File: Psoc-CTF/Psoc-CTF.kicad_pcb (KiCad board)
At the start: 2 copper layers, 100 x 100 mm, 123 parts, among them IC1 CY8C4248LQI-BL583, J1 Conn_01x02, J10 Conn_01x20, J11 Conn_01x20, J2 Conn_01x03, J3 Prog, J4 Conn_01x04, J5 USB3076-XX-X_REVC, J6 Header 9x2, J7 Header 9x2, J8 Conn_01x20, J9 Conn_01x20, P1 Power, P2 Analog, P3 Digital, P4 Digital, SW1 FSM4JSMATR, SW2 FSM4JSMATR, SW3 FSM4JSMATR, SW4 FSM4JSMATR, SW5 FSM4JSMATR, U1 AMS1117-5.0, U2 AMS1117-3.3, U3 ESP32-WROOM-32D, U4 FM24C04B-GTR, U5 CY7C65211-24LTXI, Y1 24MHz, Y2 32.768Khz

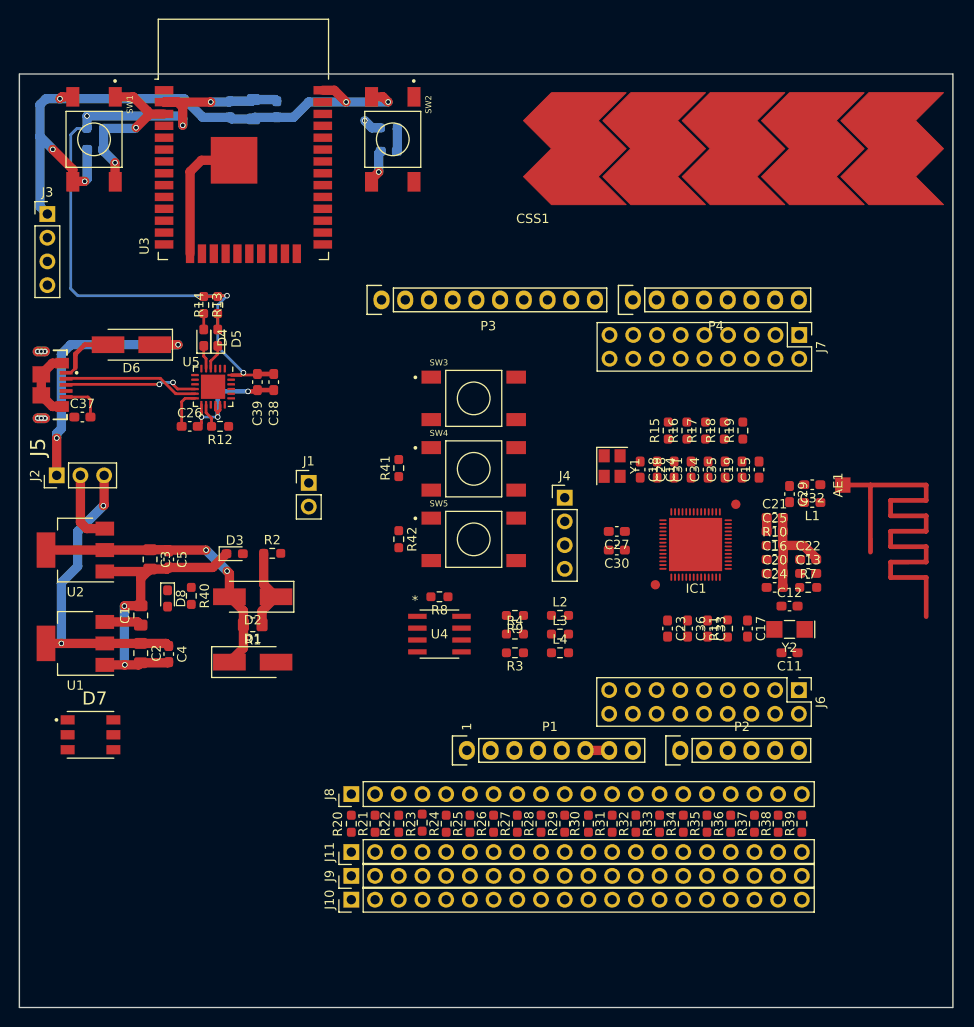
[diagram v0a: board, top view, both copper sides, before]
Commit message: Ruteo Psoc-CTF
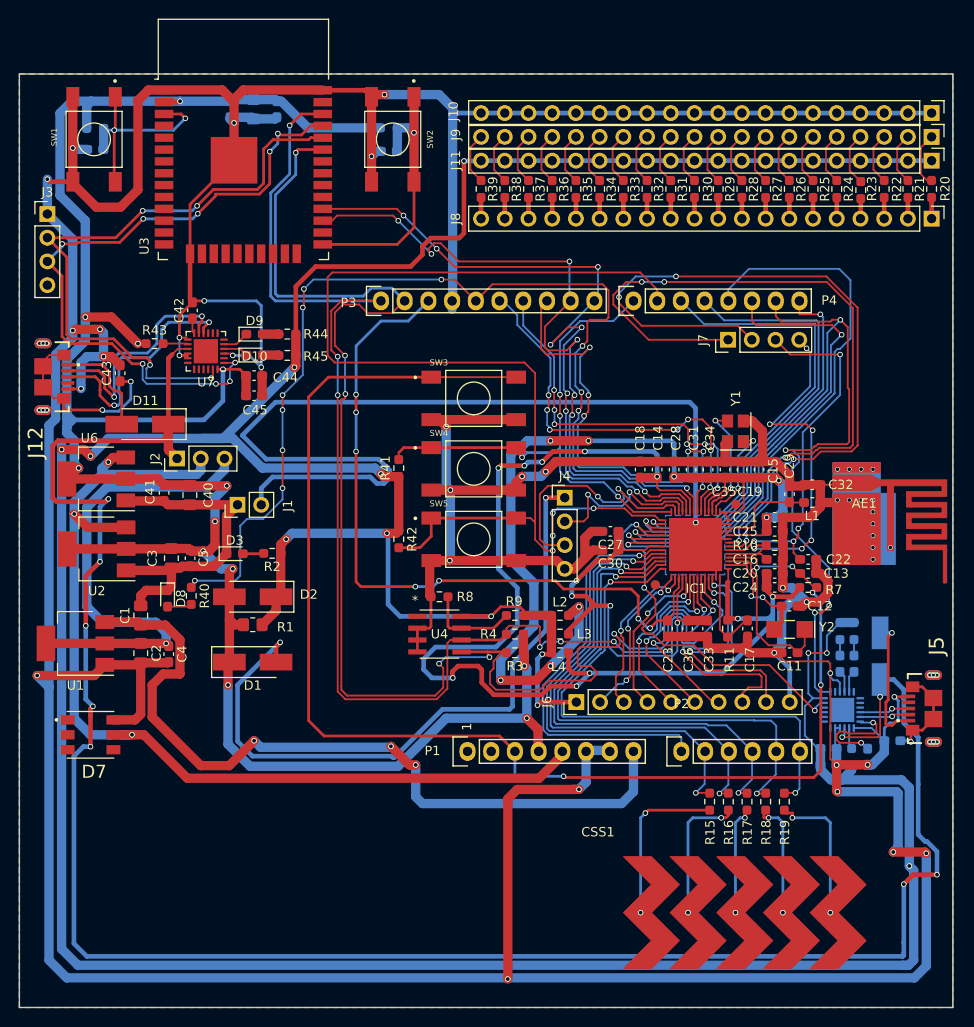
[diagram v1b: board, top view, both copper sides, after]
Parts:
- added C40: 10uF, Capacitor_SMD:C_0805_2012Metric_Pad1.18x1.45mm_HandSolder, F.Cu at (129.3, 91.5)
- added C41: 10uF, Capacitor_SMD:C_0603_1608Metric_Pad1.08x0.95mm_HandSolder, F.Cu at (126.5, 91.2)
- added C42: 1uF, Capacitor_SMD:C_0603_1608Metric_Pad1.08x0.95mm_HandSolder, F.Cu at (129.5, 71.7)
- added C43: 0.1uF, Capacitor_SMD:C_0603_1608Metric_Pad1.08x0.95mm_HandSolder, F.Cu at (121.8, 78.4)
- added C44: 1uF, Capacitor_SMD:C_0603_1608Metric_Pad1.08x0.95mm_HandSolder, F.Cu at (136.1, 78.7)
- added C45: 0.1uF, Capacitor_SMD:C_0603_1608Metric_Pad1.08x0.95mm_HandSolder, F.Cu at (136.1, 80.8)
- added D10: LED, LED_SMD:LED_0603_1608Metric_Pad1.05x0.95mm_HandSolder, F.Cu at (136.2, 76.5)
- added D11: SSA14, Diode_SMD:D_SMA_Handsoldering, F.Cu at (124.5, 83.9)
- added D9: LED, LED_SMD:LED_0603_1608Metric_Pad1.05x0.95mm_HandSolder, F.Cu at (136.2, 74.2)
- added J12: USB3076-XX-X_REVC, Psoc-CTF:microUSB, F.Cu at (113.5, 78.8)
- added R43: 10k, Resistor_SMD:R_0603_1608Metric_Pad0.98x0.95mm_HandSolder, F.Cu at (125.5, 75.2)
- added R44: 1K, Resistor_SMD:R_0603_1608Metric_Pad0.98x0.95mm_HandSolder, F.Cu at (139.7, 74.2)
- added R45: 1K, Resistor_SMD:R_0603_1608Metric_Pad0.98x0.95mm_HandSolder, F.Cu at (139.7, 76.5)
- added U6: AMS1117-3.3, Package_TO_SOT_SMD:SOT-223-3_TabPin2, F.Cu at (119.2, 89.7)
- added U7: CY7C65211-24LTXI, Package_DFN_QFN:QFN-24-1EP_4x4mm_P0.5mm_EP2.6x2.6mm, F.Cu at (131.0, 76.1)
- AE1: footprint Psoc-CTF:Antena_pad -> Psoc-CTF:Antenna_pad
- C26, C37, C38, C39, D4, D5, D6, R12, R13, R14, U5: moved to B.Cu
- J6: value Header 9x2 -> Conn_01x10; footprint Connector_PinHeader_2.54mm:PinHeader_2x09_P2.54mm_Vertical -> Connector_PinHeader_2.54mm:PinHeader_1x10_P2.54mm_Vertical
- J7: value Header 9x2 -> Conn_01x04; footprint Connector_PinHeader_2.54mm:PinHeader_2x09_P2.54mm_Vertical -> Connector_PinHeader_2.54mm:PinHeader_1x04_P2.54mm_Vertical
- moved J10 104.7 mm to (208.7, 50.6), turned to 270 degrees
- moved J5 101.7 mm to (208.9, 114.3), turned to 90 degrees
- moved J9 100.7 mm to (208.7, 53.1), turned to 270 degrees
- moved J11 96.7 mm to (208.7, 55.7), turned to 270 degrees
- moved CSS1 95.8 mm to (179.7, 139.2), turned to 0 degrees
- moved C37 93.4 mm to (204.5, 117.8), turned to 180 degrees
- moved R20 92.1 mm to (208.7, 58.7), turned to 90 degrees
- moved R21 88.8 mm to (206.2, 58.7), turned to 90 degrees
- moved J8 87.5 mm to (208.7, 61.9), turned to 270 degrees
- moved D6 86.9 mm to (203.2, 108.7), turned to 90 degrees
- moved R22 85.6 mm to (203.6, 58.7)
- moved R23 82.5 mm to (201.1, 58.8), turned to 90 degrees
- moved C26 80.8 mm to (201.9, 119.5), turned to 270 degrees
- moved R24 79.8 mm to (198.6, 58.7), turned to 90 degrees
- moved R13 77.9 mm to (200.4, 106.0)
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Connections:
- net /IOREF renamed Net-(P1-Pad2)
- net /MCU_Target/5VBUS renamed /MCU_Target/VBUS
- C6 pad 1: VDD -> +3V3
- C7 pad 1: VDD -> +3V3
- C8 pad 1: VDD -> +3V3
- IC1 pad 9: /MCU_Target/AMP_READ -> GND1
- J10 pad 1: VDD -> GND
- J10 pad 10: VDD -> GND
- J10 pad 11: VDD -> GND
- J10 pad 12: VDD -> GND
- J10 pad 13: VDD -> GND
- J10 pad 14: VDD -> GND
- J10 pad 15: VDD -> GND
- J10 pad 16: VDD -> GND
- J10 pad 17: VDD -> GND
- J10 pad 18: VDD -> GND
- J10 pad 19: VDD -> GND
- J10 pad 2: VDD -> GND
- J10 pad 20: VDD -> GND
- J10 pad 3: VDD -> GND
- J10 pad 4: VDD -> GND
- J10 pad 5: VDD -> GND
- J10 pad 6: VDD -> GND
- J10 pad 7: VDD -> GND
- J10 pad 8: VDD -> GND
- J10 pad 9: VDD -> GND
- J11 pad 1: GND -> VDD
- J11 pad 10: GND -> VDD
- J11 pad 11: GND -> VDD
- J11 pad 12: GND -> VDD
- J11 pad 13: GND -> VDD
- J11 pad 14: GND -> VDD
- J11 pad 15: GND -> VDD
- J11 pad 16: GND -> VDD
- J11 pad 17: GND -> VDD
- J11 pad 18: GND -> VDD
- J11 pad 19: GND -> VDD
- J11 pad 2: GND -> VDD
- J11 pad 20: GND -> VDD
- J11 pad 3: GND -> VDD
- J11 pad 4: GND -> VDD
- J11 pad 5: GND -> VDD
- J11 pad 6: GND -> VDD
- J11 pad 7: GND -> VDD
- J11 pad 8: GND -> VDD
- J11 pad 9: GND -> VDD
- J3 pad 2: /MONITOR/U0-TX -> /MONITOR/TXD
- J3 pad 3: /MONITOR/U0-RX -> /MONITOR/RXD
- J6 pad 1: P4.0 -> VDD
- J6 pad 10: P1.7 -> GND
- J6 pad 2: P0.0 -> P2.6
- J6 pad 3: P0.1 -> P2.7
- J6 pad 4: P0.2 -> P3.0
- J6 pad 5: P0.3 -> P3.1
- J6 pad 6: P0.4 -> P3.2
- J6 pad 7: P0.5 -> P3.3
- J6 pad 8: P0.6 -> P3.6
- J6 pad 9: P0.7 -> P3.7
- J7 pad 1: P5.0 -> P5.1
- J7 pad 2: P2.0 -> P5.0
- J7 pad 3: P2.1 -> P4.1
- J7 pad 4: P2.2 -> P4.0
- P1 pad 3: /Reset -> /MCU_Target/XRES
- P1 pad 8: /Vin -> +12V
- P2 pad 1: /A0 -> P2.0
- P2 pad 2: /A1 -> P2.1
- P2 pad 3: /A2 -> P2.2
- P2 pad 4: /A3 -> P2.3
- P2 pad 5: /A4(SDA) -> P2.4
- P2 pad 6: /A5(SCL) -> P2.5
- P3 pad 1: /A5(SCL) -> P3.5
- P3 pad 10: /8 -> P0.5
- P3 pad 2: /A4(SDA) -> P3.4
- P3 pad 3: /AREF -> /MCU_Target/VREF
- P3 pad 5: /13(SCK) -> P0.3
- P3 pad 6: /12(MISO) -> P0.1
- P3 pad 7: /11(**/MOSI) -> P0.0
- P3 pad 8: /10(**/SS) -> P0.2
- P3 pad 9: /9(**) -> P0.4
- P4 pad 1: /7 -> P1.0
- P4 pad 2: /6(**) -> P1.1
- P4 pad 3: /5(**) -> P1.2
- P4 pad 4: /4 -> P1.3
- P4 pad 5: /3(**) -> P1.7
- P4 pad 6: /2 -> P1.6
- P4 pad 7: /1(Tx) -> P1.5
- P4 pad 8: /0(Rx) -> P1.4
- R3 pad 1: VDD -> +3V3
- R4 pad 2: VDD -> +3V3
- R41 pad 2: P2.0 -> P1.0
- R42 pad 2: P2.6 -> P1.1
- R5 pad 1: VDD -> +3V3
- R6 pad 1: VDD -> +3V3
- SW4 pad 1: P2.0 -> P1.0
- SW4 pad 2: P2.0 -> P1.0
- SW5 pad 1: P2.6 -> P1.1
- SW5 pad 2: P2.6 -> P1.1
- U3 pad 2: VDD -> +3V3
- U3 pad 27: /MCU_Target/T_MCU_TX -> P0.4
- U3 pad 28: /MCU_Target/T_MCU_RX -> P0.5
- U3 pad 34: /MONITOR/U0-RX -> /MONITOR/TXD
- U3 pad 35: /MONITOR/U0-TX -> /MONITOR/RXD
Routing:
- net GND: track 206.8 -> 754.3 mm, vias 11 -> 46
- net VDD: track 93.6 -> 412.5 mm, vias 6 -> 13
- net +3V3: track 31.6 -> 233.3 mm, vias 2 -> 12
- net /MCU_Target/VBUS: track 28.6 -> 225.3 mm, vias 2 -> 9
- net P3.4: track 0.00 -> 158.2 mm, vias 0 -> 7
- net /MCU_Target/XRES: track 0.00 -> 148.6 mm, vias 0 -> 5
- net P3.5: track 0.00 -> 145.1 mm, vias 0 -> 7
- net /MCU_Target/VDDD: track 0.00 -> 127.9 mm, vias 0 -> 10
- net P1.1: track 0.00 -> 122.9 mm, vias 0 -> 4
- net GND1: track 0.00 -> 114.8 mm, vias 0 -> 1
- net P0.3: track 0.00 -> 113.6 mm, vias 0 -> 12
- net P1.5: track 0.00 -> 101.6 mm, vias 0 -> 5
- net +5V: track 7.92 -> 107.7 mm, vias 0 -> 3
- net /MCU_Target/VDDR: track 1.50 -> 98.1 mm, vias 0 -> 8
- net P1.4: track 0.00 -> 82.8 mm, vias 0 -> 4
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- added copper zone on B.Cu, net GND
- added copper zone on F.Cu, net GND
- added copper zone on B.Cu, net GND1
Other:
- net class Default: clearance 0.2 -> 0.19; trace_width 0.25 -> 0.2
- net class Power added: clearance 0.2, trace_width 1, via_dia 0.6, via_drill 0.4
- rule trace_clearance: 0.2 -> 0.19
